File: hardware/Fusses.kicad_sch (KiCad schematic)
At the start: 3 parts

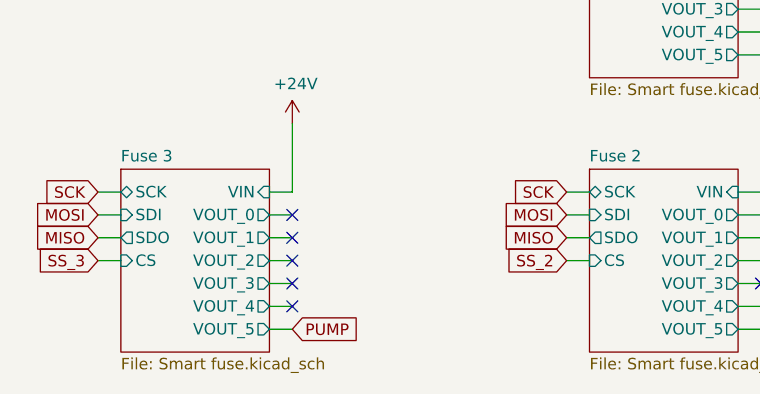
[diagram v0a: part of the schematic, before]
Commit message: minor improvements
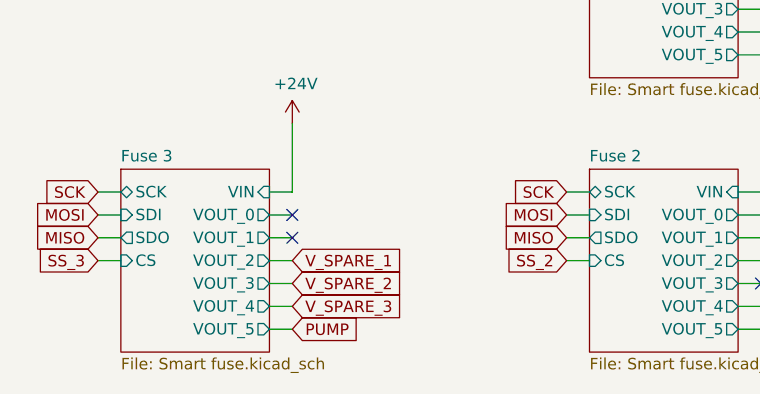
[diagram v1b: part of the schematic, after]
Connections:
- no-connect marks 6 -> 3
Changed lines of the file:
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@@
   )
   (no_connect (at 129.54 137.922))
-  (no_connect (at 77.47 140.462))
-  (no_connect (at 77.47 135.382))
   (no_connect (at 77.47 132.842))
   (no_connect (at 77.47 130.302))
-  (no_connect (at 77.47 137.922))
   (wire (pts (xy 242.824 114.3) (xy 245.364 114.3))
     (stroke (width 0) (type default) (color 0 0 0 0))
@@
     )
   )
+  (global_label "V_SPARE_3" (shape input) (at 77.47 140.462 0) (fields_autoplaced)
+    (effects (font (size 1.27 1.27)) (justify left))
+    (property "Intersheet References" "${INTERSHEET_REFS}" (id 0) (at 90.0147 140.3826 0)
+      (effects (font (size 1.27 1.27)) (justify left) hide)
+    )
+  )
+  (global_label "V_SPARE_1" (shape input) (at 77.47 135.382 0) (fields_autoplaced)
+    (effects (font (size 1.27 1.27)) (justify left))
+    (property "Intersheet References" "${INTERSHEET_REFS}" (id 0) (at 90.0147 135.3026 0)
+      (effects (font (size 1.27 1.27)) (justify left) hide)
+    )
+  )
   (global_label "FAN_L" (shape input) (at 132.08 107.442 0) (fields_autoplaced)
     (effects (font (size 1.27 1.27)) (justify left))
@@
     )
   )
+  (global_label "V_SPARE_2" (shape input) (at 77.47 137.922 0) (fields_autoplaced)
+    (effects (font (size 1.27 1.27)) (justify left))
+    (property "Intersheet References" "${INTERSHEET_REFS}" (id 0) (at 90.0147 137.8426 0)
+      (effects (font (size 1.27 1.27)) (justify left) hide)
+    )
+  )
